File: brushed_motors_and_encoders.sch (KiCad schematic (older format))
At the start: 26 parts, among them J301 M0_CONN, J302 M1_CONN, J303 M2_CONN, J304 M3_CONN, J305 E0_CONN, J306 E1_CONN, J307 E2_CONN, J308 E3_CONN, J309 V Encoders jamper, J310 V Encoders external, U301 DRV8871DDA, U302 DRV8871DDA, U303 DRV8871DDA, U304 DRV8871DDA

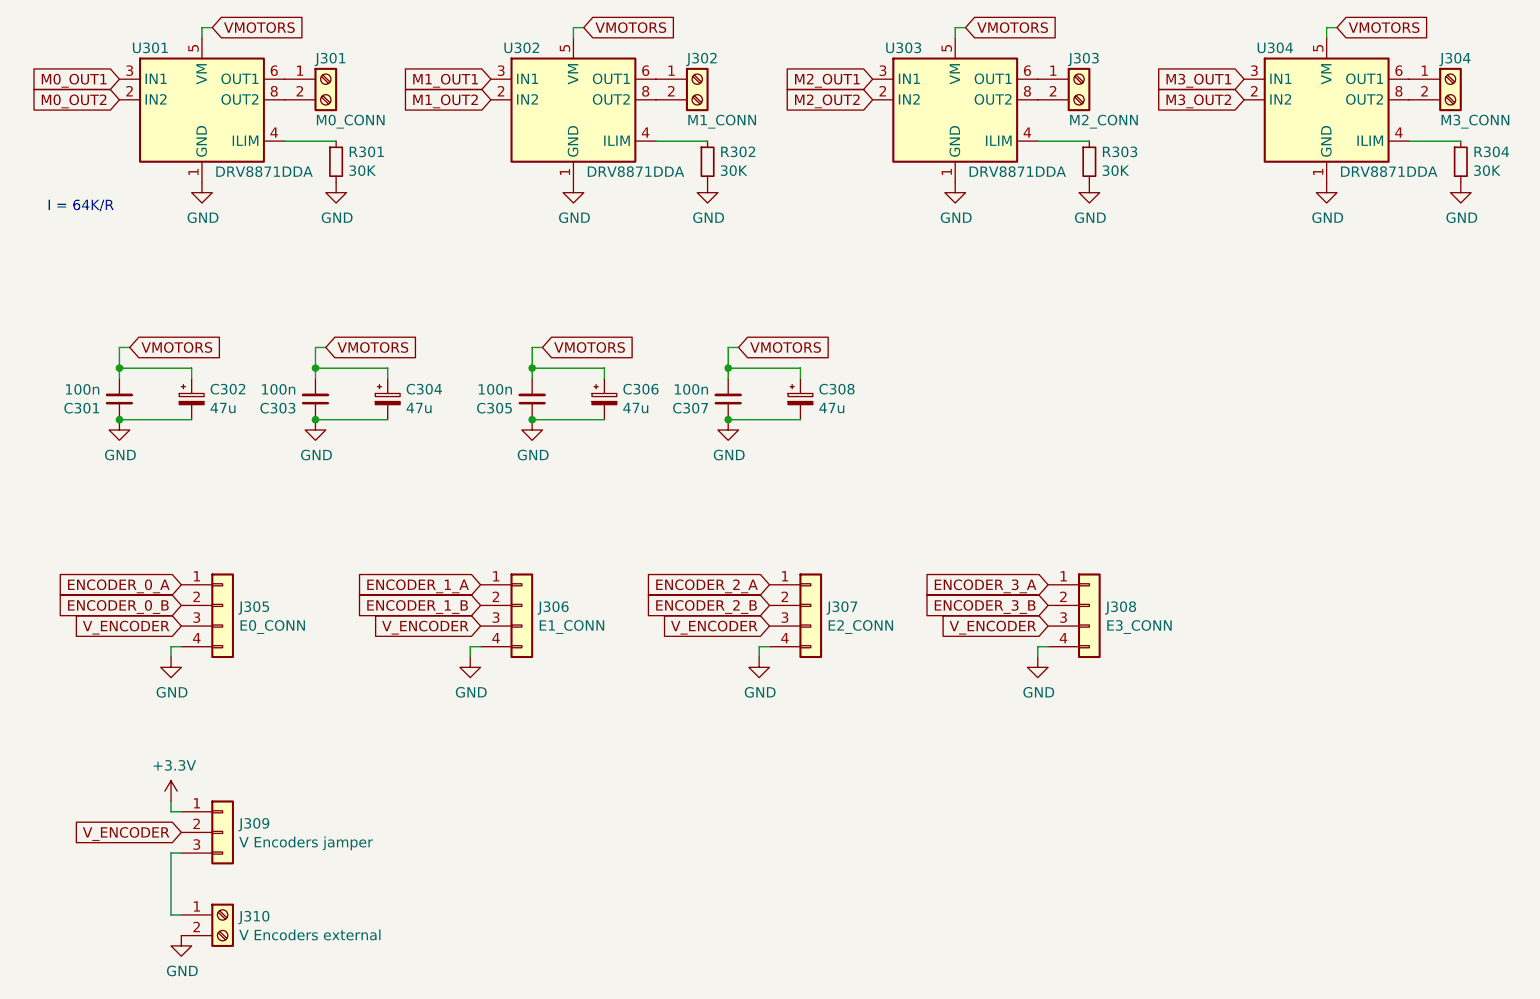
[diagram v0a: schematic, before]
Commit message: Layout
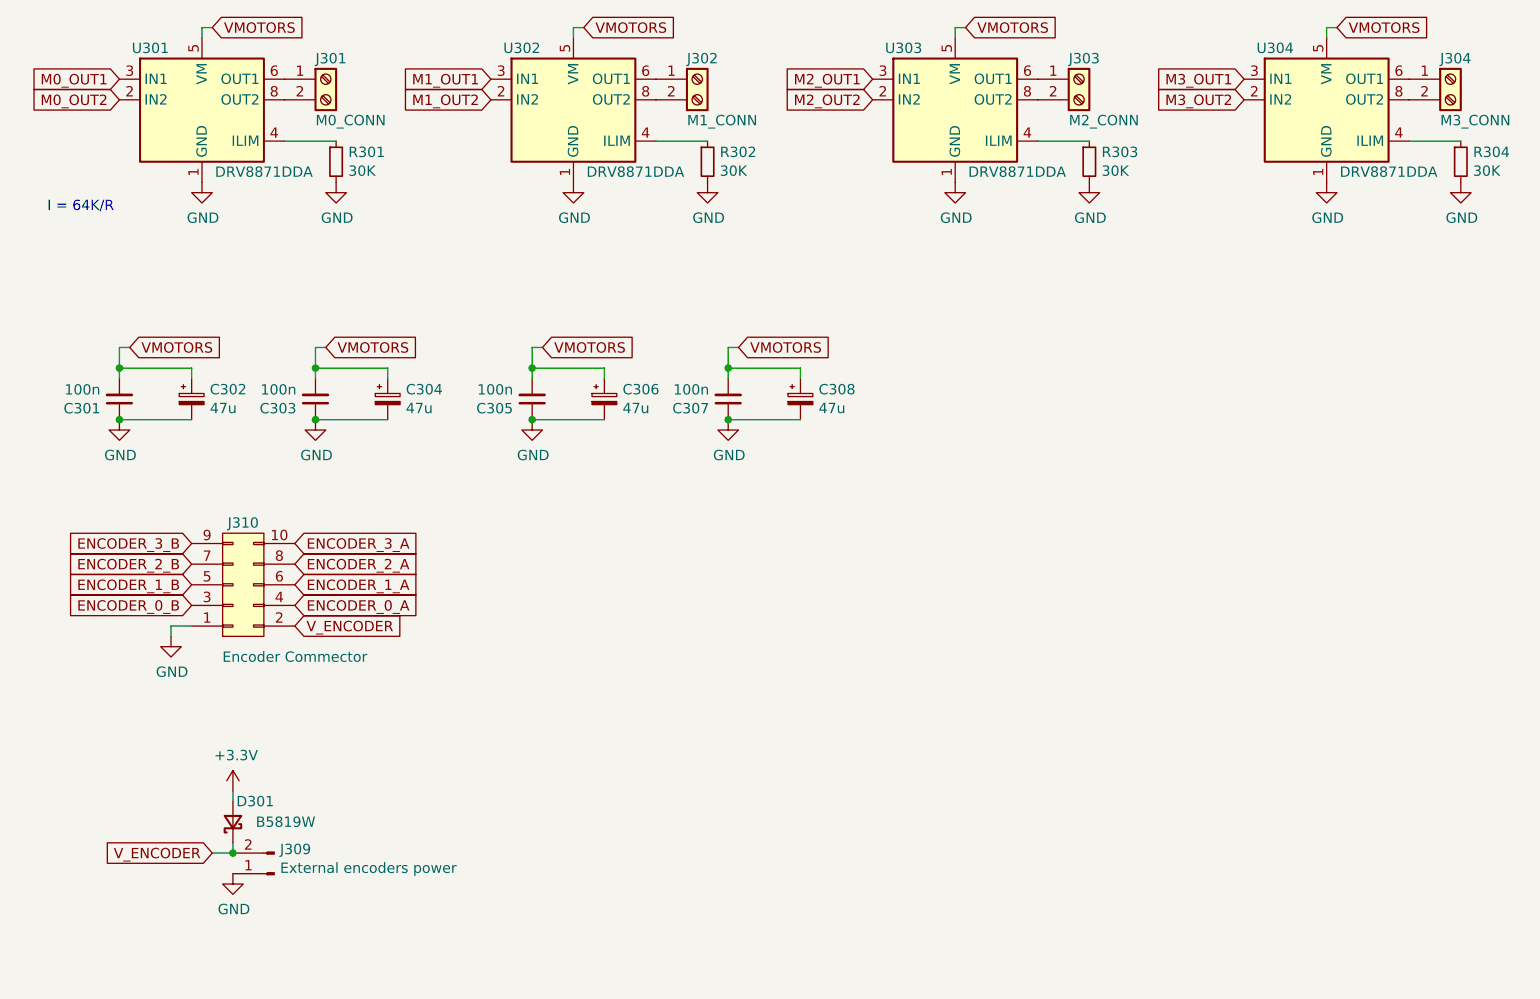
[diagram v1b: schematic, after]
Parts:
- removed J305: E0_CONN, symbol Connector_Generic:Conn_01x04
- removed J306: E1_CONN, symbol Connector_Generic:Conn_01x04
- removed J307: E2_CONN, symbol Connector_Generic:Conn_01x04
- removed J308: E3_CONN, symbol Connector_Generic:Conn_01x04
- removed J309: V Encoders jamper, symbol Connector_Generic:Conn_01x03
- removed J310: V Encoders external, VsReality_Footprints:DB128L_5.08_2P_GN_S, symbol Connector:Screw_Terminal_01x02
- added D301: B5819W, Diode_SMD:D_SOD-123, symbol Device:D_Schottky_Small
- added J309: External encoders power, Connector_PinHeader_2.54mm:PinHeader_1x02_P2.54mm_Vertical, symbol Connector:Conn_01x02_Male
- added J310: Encoder Commector, VsReality_Footprints:Encoder_PinHeader_4x04_P2.54mm_Vertical, symbol VsReality_Symbols:EncoderPinHeaderConnector_04
- J301, J302, J303, J304: footprint VsReality_Footprints:DB128L_5.08_2P_GN_S -> VsReality_Footprints:Ningbo_Kangnex_Elec_WJ128V_5_0_2P
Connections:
- net +3V3: now also D301.2 (A)
- net ENCODER_0_A: now also J310.4 (Pin_4)
- net ENCODER_0_B: now also J310.3 (Pin_3)
- net ENCODER_1_A: now also J310.6 (Pin_6)
- net ENCODER_1_B: now also J310.5 (Pin_5)
- net ENCODER_2_A: now also J310.8 (Pin_8)
- net ENCODER_2_B: now also J310.7 (Pin_7)
- net ENCODER_3_A: now also J310.10 (Pin_10)
- net ENCODER_3_B: now also J310.9 (Pin_9)
- net GND: now also J309.1 (Pin_1), J310.1 (GND)
- net V_ENCODER: now also D301.1 (K), J309.2 (Pin_2), J310.2 (Power)
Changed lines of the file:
@@
 F 0 "J304" H 9050 1850 50  0000 L CNN
 F 1 "M3_CONN" H 9050 1550 50  0000 L CNN
-F 2 "VsReality_Footprints:DB128L_5.08_2P_GN_S" H 9100 1750 50  0001 C CNN
+F 2 "VsReality_Footprints:Ningbo_Kangnex_Elec_WJ128V_5_0_2P" H 9100 1750 50  0001 C CNN
 F 3 "~" H 9100 1750 50  0001 C CNN
 	1    9100 1750
@@
 F 0 "J303" H 7250 1850 50  0000 L CNN
 F 1 "M2_CONN" H 7250 1550 50  0000 L CNN
-F 2 "VsReality_Footprints:DB128L_5.08_2P_GN_S" H 7300 1750 50  0001 C CNN
+F 2 "VsReality_Footprints:Ningbo_Kangnex_Elec_WJ128V_5_0_2P" H 7300 1750 50  0001 C CNN
 F 3 "~" H 7300 1750 50  0001 C CNN
 	1    7300 1750
@@
 F 0 "J302" H 5400 1850 50  0000 L CNN
 F 1 "M1_CONN" H 5400 1550 50  0000 L CNN
-F 2 "VsReality_Footprints:DB128L_5.08_2P_GN_S" H 5450 1750 50  0001 C CNN
+F 2 "VsReality_Footprints:Ningbo_Kangnex_Elec_WJ128V_5_0_2P" H 5450 1750 50  0001 C CNN
 F 3 "~" H 5450 1750 50  0001 C CNN
 	1    5450 1750
@@
 F 0 "J301" H 3600 1850 50  0000 L CNN
 F 1 "M0_CONN" H 3600 1550 50  0000 L CNN
-F 2 "VsReality_Footprints:DB128L_5.08_2P_GN_S" H 3650 1750 50  0001 C CNN
+F 2 "VsReality_Footprints:Ningbo_Kangnex_Elec_WJ128V_5_0_2P" H 3650 1750 50  0001 C CNN
 F 3 "~" H 3650 1750 50  0001 C CNN
 	1    3650 1750
@@
 	1    0    0    -1
 $EndComp
-Wire Wire Line
-	2900 4500 2900 4550
-Wire Wire Line
-	2950 4500 2900 4500
-$Comp
-L power:GND #PWR0313
-U 1 1 60AA39E0
-P 2900 4550
-F 0 "#PWR0313" H 2900 4300 50  0001 C CNN
-F 1 "GND" H 2905 4377 50  0000 C CNN
-F 2 "" H 2900 4550 50  0001 C CNN
-F 3 "" H 2900 4550 50  0001 C CNN
-	1    2900 4550
-	1    0    0    -1
-$EndComp
-Text GLabel 2950 4400 0    50   Input ~ 0
+$Comp
+L Connector:Conn_01x02_Male J309
+U 1 1 60C2A5CF
+P 3400 5600
+F 0 "J309" H 3372 5482 50  0000 R CNN
+F 1 "External encoders power" H 3372 5573 50  0000 R CNN
+F 2 "Connector_PinHeader_2.54mm:PinHeader_1x02_P2.54mm_Vertical" H 3400 5600 50  0001 C CNN
+F 3 "~" H 3400 5600 50  0001 C CNN
+	1    3400 5600
+	-1   0    0    1
+$EndComp
+$Comp
+L power:GND #PWR0118
+U 1 1 60C31896
+P 3200 5600
+F 0 "#PWR0118" H 3200 5350 50  0001 C CNN
+F 1 "GND" H 3205 5427 50  0000 C CNN
+F 2 "" H 3200 5600 50  0001 C CNN
+F 3 "" H 3200 5600 50  0001 C CNN
+	1    3200 5600
+	1    0    0    -1
+$EndComp
+Text GLabel 3100 5500 0    50   Input ~ 0
 V_ENCODER
-Text GLabel 2950 4300 0    50   Input ~ 0
+$Comp
+L power:+3.3V #PWR0119
+U 1 1 60C335D0
+P 3200 5200
+F 0 "#PWR0119" H 3200 5050 50  0001 C CNN
+F 1 "+3.3V" H 3215 5373 50  0000 C CNN
+F 2 "" H 3200 5200 50  0001 C CNN
+F 3 "" H 3200 5200 50  0001 C CNN
+	1    3200 5200
+	1    0    0    -1
+$EndComp
+$Comp
+L Device:D_Schottky_Small D?
+U 1 1 60C368EC
+P 3200 5350
+AR Path="/60C368EC" Ref="D?"  Part="1"
+AR Path="/60A3E5C0/60C368EC" Ref="D301"  Part="1"
+F 0 "D301" V 3300 5150 50  0000 L CNN
+F 1 "B5819W" V 3200 4950 50  0000 L CNN
+F 2 "Diode_SMD:D_SOD-123" V 3200 5350 50  0001 C CNN
+F 3 "~" V 3200 5350 50  0001 C CNN
+F 4 "C8598" H 3200 5350 50  0001 C CNN "LCSC Part #"
+	1    3200 5350
+	0    -1   -1   0
+$EndComp
+Wire Wire Line
+	3200 5200 3200 5250
+Wire Wire Line
+	3200 5450 3200 5500
+Wire Wire Line
+	3100 5500 3200 5500
+Connection ~ 3200 5500
+$Comp
+L power:GND #PWR0120
+U 1 1 60C2E84F
+P 2900 4450
+F 0 "#PWR0120" H 2900 4200 50  0001 C CNN
+F 1 "GND" H 2905 4277 50  0000 C CNN
+F 2 "" H 2900 4450 50  0001 C CNN
+F 3 "" H 2900 4450 50  0001 C CNN
+	1    2900 4450
+	1    0    0    -1
+$EndComp
+Text GLabel 3500 4400 2    50   Input ~ 0
+V_ENCODER
+Text GLabel 3500 4300 2    50   Input ~ 0
+ENCODER_0_A
+Text GLabel 3000 4300 0    50   Input ~ 0
 ENCODER_0_B
-Text GLabel 2950 4200 0    50   Input ~ 0
-ENCODER_0_A
-$Comp
-L Connector_Generic:Conn_01x04 J305
-U 1 1 60A63E75
-P 3150 4300
-F 0 "J305" H 3230 4292 50  0000 L CNN
-F 1 "E0_CONN" H 3230 4201 50  0000 L CNN
-F 2 "" H 3150 4300 50  0001 C CNN
-F 3 "~" H 3150 4300 50  0001 C CNN
-	1    3150 4300
-	1    0    0    -1
-$EndComp
-Wire Wire Line
-	4350 4500 4350 4550
-Wire Wire Line
-	4400 4500 4350 4500
-$Comp
-L power:GND #PWR0314
-U 1 1 60AA86E4
-P 4350 4550
-F 0 "#PWR0314" H 4350 4300 50  0001 C CNN
-F 1 "GND" H 4355 4377 50  0000 C CNN
-F 2 "" H 4350 4550 50  0001 C CNN
-F 3 "" H 4350 4550 50  0001 C CNN
-	1    4350 4550
-	1    0    0    -1
-$EndComp
-Text GLabel 4400 4400 0    50   Input ~ 0
-V_ENCODER
-Text GLabel 4400 4300 0    50   Input ~ 0
+Text GLabel 3500 4200 2    50   Input ~ 0
+ENCODER_1_A
+Text GLabel 3000 4200 0    50   Input ~ 0
 ENCODER_1_B
-Text GLabel 4400 4200 0    50   Input ~ 0
-ENCODER_1_A
-$Comp
-L Connector_Generic:Conn_01x04 J306
-U 1 1 60AA86ED
-P 4600 4300
-F 0 "J306" H 4680 4292 50  0000 L CNN
-F 1 "E1_CONN" H 4680 4201 50  0000 L CNN
-F 2 "" H 4600 4300 50  0001 C CNN
-F 3 "~" H 4600 4300 50  0001 C CNN
-	1    4600 4300
-	1    0    0    -1
-$EndComp
-Wire Wire Line
-	5750 4500 5750 4550
-Wire Wire Line
-	5800 4500 5750 4500
-$Comp
-L power:GND #PWR0315
-U 1 1 60AA96F0
-P 5750 4550
-F 0 "#PWR0315" H 5750 4300 50  0001 C CNN
-F 1 "GND" H 5755 4377 50  0000 C CNN
-F 2 "" H 5750 4550 50  0001 C CNN
-F 3 "" H 5750 4550 50  0001 C CNN
-	1    5750 4550
-	1    0    0    -1
-$EndComp
-Text GLabel 5800 4400 0    50   Input ~ 0
-V_ENCODER
-Text GLabel 5800 4300 0    50   Input ~ 0
+Text GLabel 3500 4100 2    50   Input ~ 0
+ENCODER_2_A
+Text GLabel 3000 4100 0    50   Input ~ 0
 ENCODER_2_B
-Text GLabel 5800 4200 0    50   Input ~ 0
-ENCODER_2_A
-$Comp
-L Connector_Generic:Conn_01x04 J307
-U 1 1 60AA96F9
-P 6000 4300
-F 0 "J307" H 6080 4292 50  0000 L CNN
-F 1 "E2_CONN" H 6080 4201 50  0000 L CNN
-F 2 "" H 6000 4300 50  0001 C CNN
-F 3 "~" H 6000 4300 50  0001 C CNN
-	1    6000 4300
-	1    0    0    -1
-$EndComp
-Wire Wire Line
-	7100 4500 7100 4550
-Wire Wire Line
-	7150 4500 7100 4500
-$Comp
-L power:GND #PWR0316
-U 1 1 60AAAC83
-P 7100 4550
-F 0 "#PWR0316" H 7100 4300 50  0001 C CNN
-F 1 "GND" H 7105 4377 50  0000 C CNN
-F 2 "" H 7100 4550 50  0001 C CNN
-F 3 "" H 7100 4550 50  0001 C CNN
-	1    7100 4550
-	1    0    0    -1
-$EndComp
-Text GLabel 7150 4400 0    50   Input ~ 0
-V_ENCODER
-Text GLabel 7150 4300 0    50   Input ~ 0
+Text GLabel 3500 4000 2    50   Input ~ 0
+ENCODER_3_A
+Text GLabel 3000 4000 0    50   Input ~ 0
 ENCODER_3_B
-Text GLabel 7150 4200 0    50   Input ~ 0
-ENCODER_3_A
-$Comp
-L Connector_Generic:Conn_01x04 J308
-U 1 1 60AAAC8C
-P 7350 4300
-F 0 "J308" H 7430 4292 50  0000 L CNN
-F 1 "E3_CONN" H 7430 4201 50  0000 L CNN
-F 2 "" H 7350 4300 50  0001 C CNN
-F 3 "~" H 7350 4300 50  0001 C CNN
-	1    7350 4300
-	1    0    0    -1
-$EndComp
-$Comp
-L Connector_Generic:Conn_01x03 J309
-U 1 1 60A25E97
-P 3150 5400
-F 0 "J309" H 3230 5442 50  0000 L CNN
-F 1 "V Encoders jamper" H 3230 5351 50  0000 L CNN
-F 2 "" H 3150 5400 50  0001 C CNN
-F 3 "~" H 3150 5400 50  0001 C CNN
-	1    3150 5400
-	1    0    0    -1
-$EndComp
-Text GLabel 2950 5400 0    50   Input ~ 0
-V_ENCODER
-$Comp
-L power:+3.3V #PWR0317
-U 1 1 60A28183
-P 2900 5250
-F 0 "#PWR0317" H 2900 5100 50  0001 C CNN
-F 1 "+3.3V" H 2915 5423 50  0000 C CNN
-F 2 "" H 2900 5250 50  0001 C CNN
-F 3 "" H 2900 5250 50  0001 C CNN
-	1    2900 5250
-	1    0    0    -1
-$EndComp
-Wire Wire Line
-	2900 5250 2900 5300
-Wire Wire Line
-	2900 5300 2950 5300
-$Comp
-L Connector:Screw_Terminal_01x02 J?
-U 1 1 60A2D1AA
-P 3150 5800
-AR Path="/60A2D1AA" Ref="J?"  Part="1"
-AR Path="/60A3E5C0/60A2D1AA" Ref="J310"  Part="1"
-F 0 "J310" H 3230 5792 50  0000 L CNN
-F 1 "V Encoders external" H 3230 5701 50  0000 L CNN
-F 2 "VsReality_Footprints:DB128L_5.08_2P_GN_S" H 3150 5800 50  0001 C CNN
-F 3 "~" H 3150 5800 50  0001 C CNN
-	1    3150 5800
-	1    0    0    -1
-$EndComp
-$Comp
-L power:GND #PWR?
-U 1 1 60A2D1B6
-P 2950 5900
-AR Path="/60A2D1B6" Ref="#PWR?"  Part="1"
-AR Path="/60A3E5C0/60A2D1B6" Ref="#PWR0318"  Part="1"
-F 0 "#PWR0318" H 2950 5650 50  0001 C CNN
-F 1 "GND" H 2955 5727 50  0000 C CNN
-F 2 "" H 2950 5900 50  0001 C CNN
-F 3 "" H 2950 5900 50  0001 C CNN
-	1    2950 5900
-	1    0    0    -1
-$EndComp
-Wire Wire Line
-	2950 5500 2900 5500
-Wire Wire Line
-	2900 5500 2900 5800
-Wire Wire Line
-	2900 5800 2950 5800
+Wire Wire Line
+	2900 4450 2900 4400
+Wire Wire Line
+	2900 4400 3000 4400
+$Comp
+L VsReality_Symbols:EncoderPinHeaderConnector_04 J310
+U 1 1 60C2E219
+P 3200 4300
+F 0 "J310" H 3250 3900 50  0000 C CNN
+F 1 "Encoder Commector" H 3500 4550 50  0000 C CNN
+F 2 "VsReality_Footprints:Encoder_PinHeader_4x04_P2.54mm_Vertical" H 3200 4300 50  0001 C CNN
+F 3 "~" H 3200 4300 50  0001 C CNN
+	1    3200 4300
+	1    0    0    1
+$EndComp
 $EndSCHEMATC
